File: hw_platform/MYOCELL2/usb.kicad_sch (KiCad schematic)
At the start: 12 parts, among them J4 USB_B_Micro, Q1 MBT3904DW1, U5 CP2104

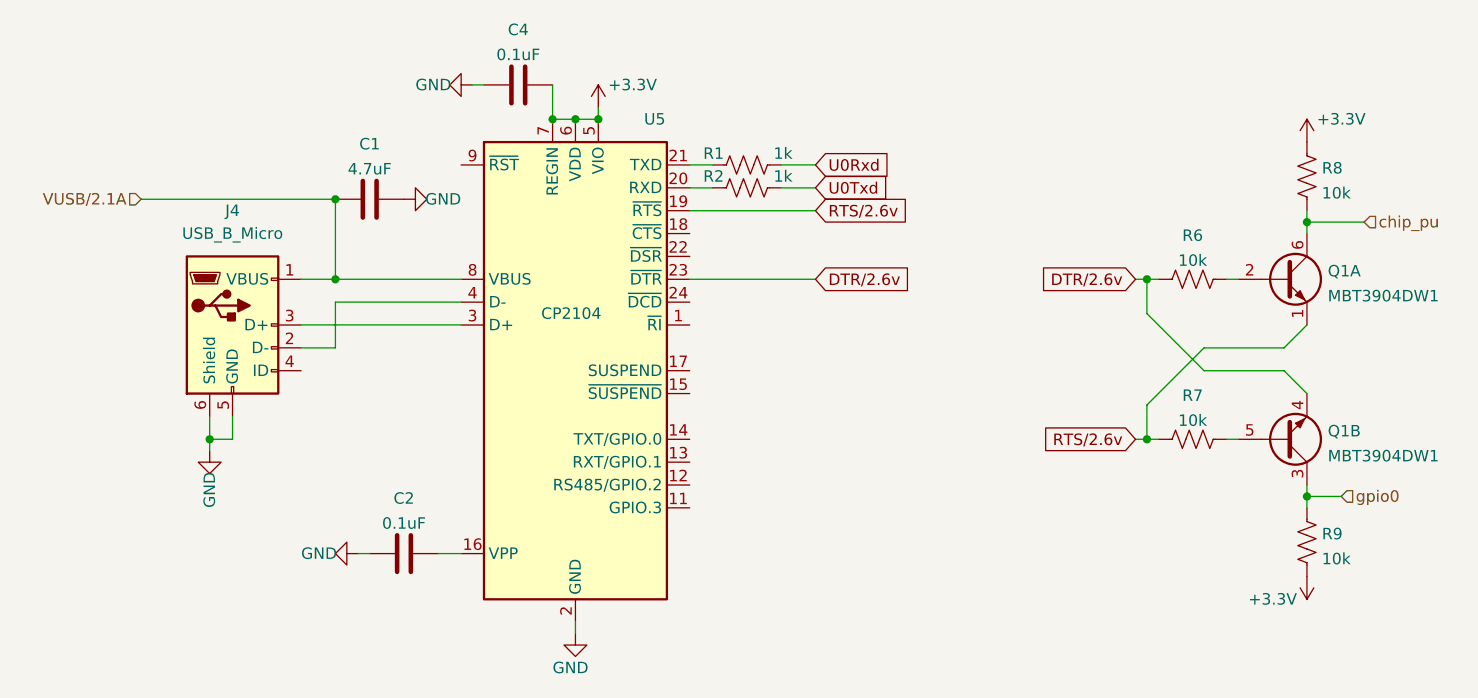
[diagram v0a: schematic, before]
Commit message: working on schematic:
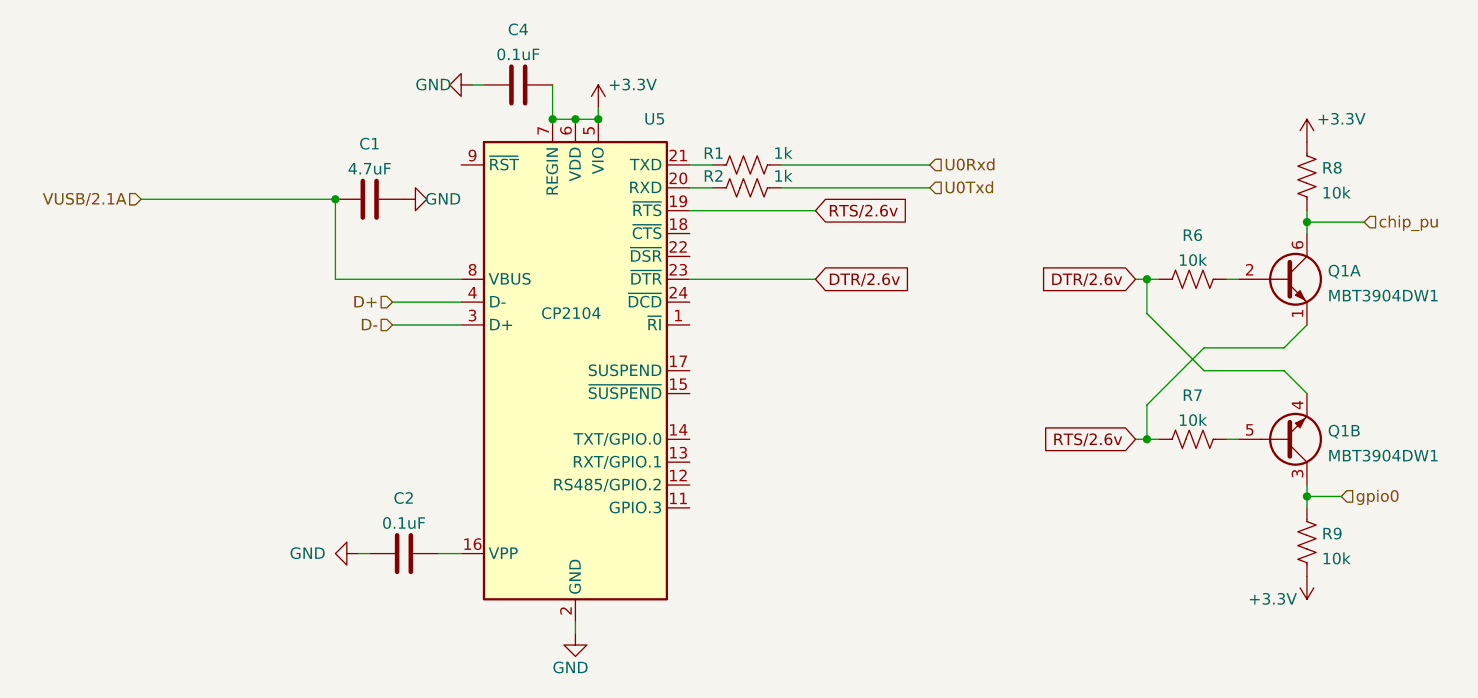
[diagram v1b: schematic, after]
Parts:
- removed J4: USB_B_Micro, Connector_USB:USB3_Micro-B_Connfly_DS1104-01, symbol Connector:USB_B_Micro
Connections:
- net D-: now reaches U5.3 (D+)
- net D+: now reaches U5.4 (D-)
